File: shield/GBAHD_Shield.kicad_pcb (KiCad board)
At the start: 2 copper layers, 53.4 x 53.1 mm, 38 parts, among them J1 Conn_01x01, J10 Conn_01x10, J11 Conn_02x03_Odd_Even, J12 Conn_01x01, J2 FFC_OGBA_32, J3 FFC_GBA-SP, J4 Conn_01x16, J5 FFC_OGBA_40, J6 Conn_01x06, J7 Conn_01x08, J8 Conn_01x10, J9 Conn_01x08, Q1 Q_PMOS_GSD, SW1 SW_Push, T1 Conn_01x01, T2 Conn_01x01, T3 Conn_01x01, T4 Conn_01x01, T5 Conn_01x01, T6 Conn_01x01, T7 Conn_01x01, T8 Conn_01x01, U1 AZ1117R-ADJ, U2 74HC595, U3 74HC595, U4 SNES_7PIN, U5 ATmega328P-AU

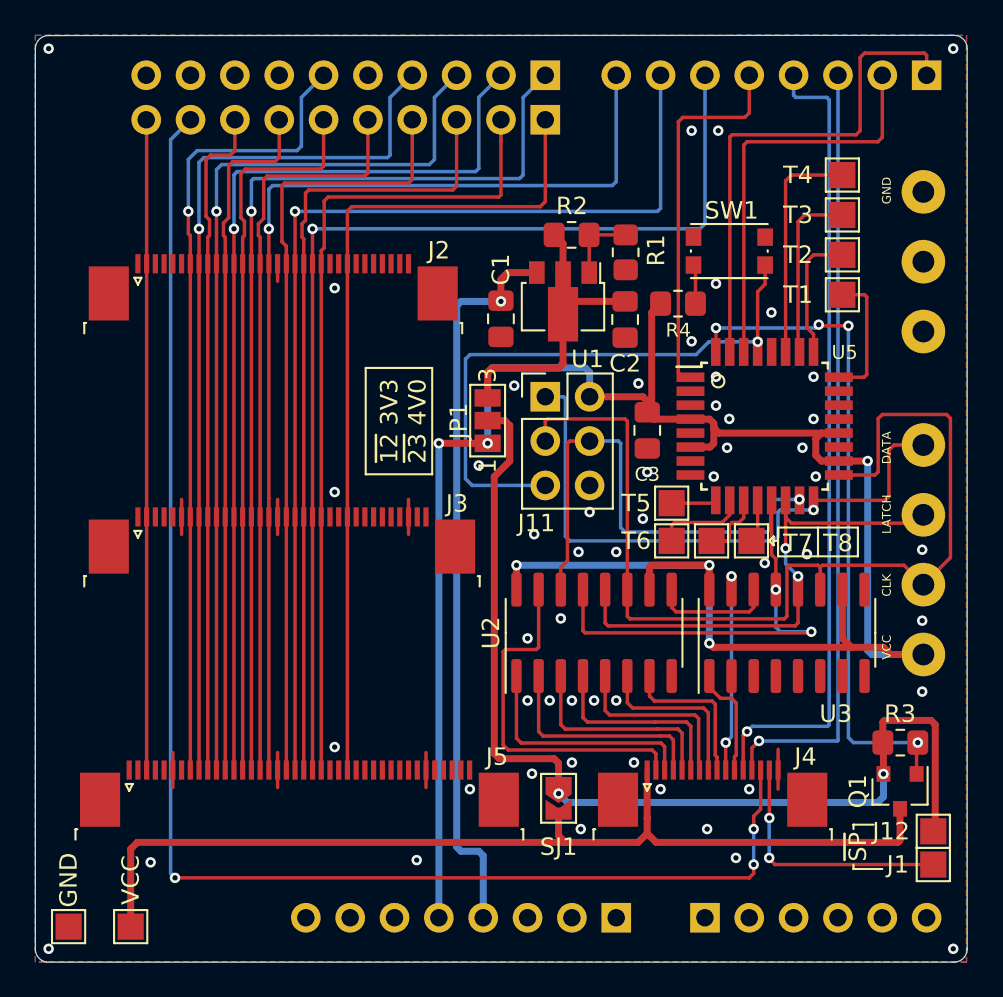
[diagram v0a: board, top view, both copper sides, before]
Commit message: Develop (#16)
* Remove get_components from Makefile, fix bluepad path

* Fixed naming of submodule

* Fixed submodule mess

* Removed bluepad32

* Re-Add Bluepad32 properly

* Update Build for adding web/bitstream handler

* Add implementation for web handler and bitstream handler

* Update arduino version

* Fix build by using bluepad template as component foundation

* Removed bluepad submodule

* Copying default component files

* Remove get_components

* Improved over all build config

* Overall refactoring and added wifi and mega handler

* Minor updates to sdkconfig

* Add first crude version to update firmware

* Remove Bluepad Debug outputs

* some cleanup

* updated .gitignore and added some files

* updated gitmodules

* fixed submodules

* Update Upgrade function

* Fix gitignore

* Fix SPIFFS upload

* a little bit of tinkering

* Changed order of run/init to be faster for TWI

* Removed endTransmission after requestFrom

* changed twi handling

* added definition for bigger I2C-Buffer

* some cleanup

* remove wifi

* Fix sending of inputs without controller available

* Fix WiFi

* fixed button mapping

* fixed button mappings and polling intervalls

* Improve Timer Code

* Refactoring and Preferences

* Add Prefs

* Add prefs

* fixed verify_flash() --> missing beginTransmission()

* Added Bluetooth Mapping, Preferences Refactoring

* Add bluetooth cfg

* Refactoring

* Remove template

* CMake fixes

* changed TWI handling - added data validity timeout

* some cleanup

* Added License Hadder

* updated CPU-flex

* Refactoring

* Beautifying

* Update Bitstream

* refactored avr-firmware to be makefile project

* added controller detection

* Better layout

* Better shield handling

* Better OTA

* For now - only load bitstream from SPIFFS to be faster

* Add Force option for ATMega update

* Added Force Option for Mega Update

* Upd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
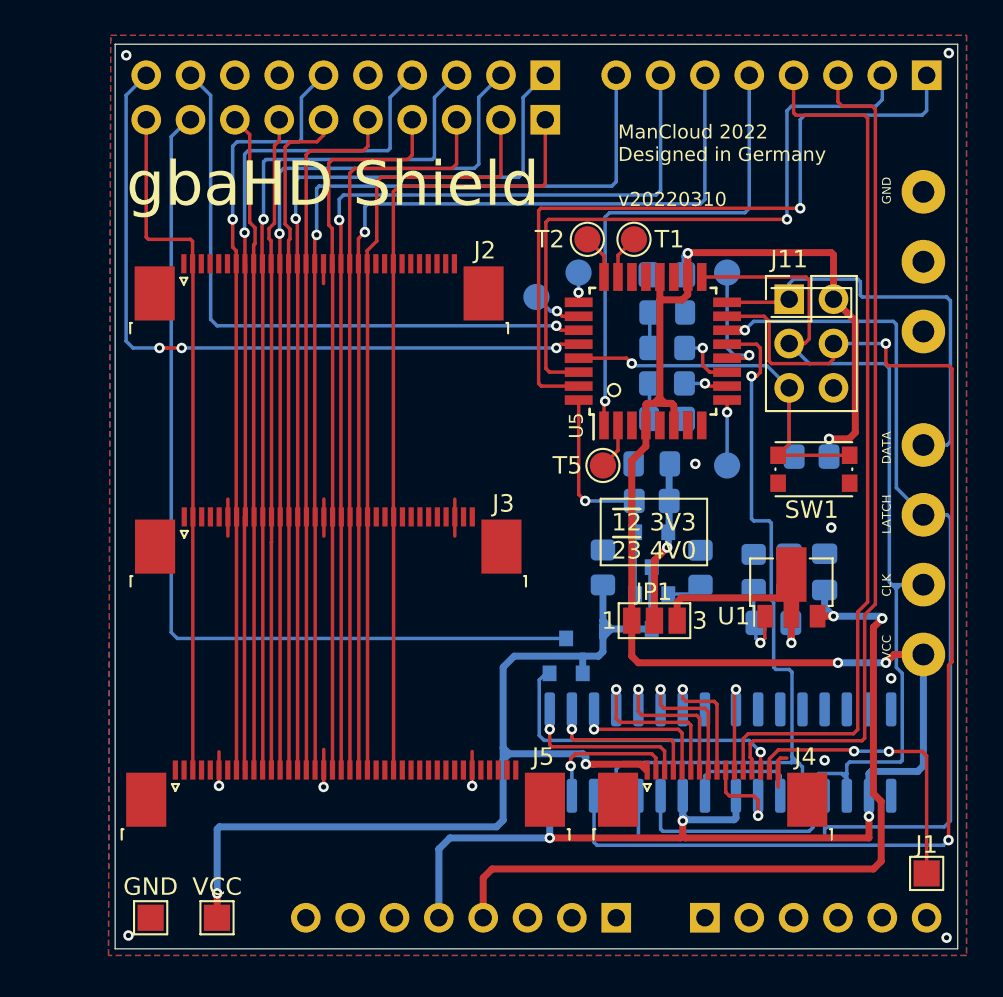
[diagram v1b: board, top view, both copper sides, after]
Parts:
- removed GND, J12, T8, VCC: Conn_01x01, TestPoint:TestPoint_Pad_1.5x1.5mm
- removed SJ1: SOLDER_JUMPER, Jumper:SolderJumper-2_P1.3mm_Open_TrianglePad1.0x1.5mm
- added C4: 47uF, Capacitor_SMD:C_0805_2012Metric_Pad1.18x1.45mm_HandSolder, B.Cu at (74.9, 51.0)
- added D1: RED, LED_SMD:LED_0805_2012Metric_Pad1.15x1.40mm_HandSolder, B.Cu at (75.8, 48.4)
- added D2: GREEN, LED_SMD:LED_0805_2012Metric_Pad1.15x1.40mm_HandSolder, B.Cu at (75.8, 42.3)
- added GND1: Conn_01x01, TestPoint:TestPoint_Pad_1.5x1.5mm, F.Cu at (46.2, 77.0)
- added Q2: Q_NMOS_GSD, Package_TO_SOT_SMD:SOT-23, B.Cu at (74.9, 59.4)
- added Q3: Q_NMOS_GSD, Package_TO_SOT_SMD:SOT-23, B.Cu at (70.0, 62.0)
- added R5: 500, Resistor_SMD:R_0805_2012Metric_Pad1.20x1.40mm_HandSolder, B.Cu at (77.7, 56.9)
- added R6: 1k, Resistor_SMD:R_0805_2012Metric_Pad1.20x1.40mm_HandSolder, B.Cu at (75.8, 46.4)
- added R7: 1k, Resistor_SMD:R_0805_2012Metric_Pad1.20x1.40mm_HandSolder, B.Cu at (75.8, 44.3)
- added R8: 10K, Resistor_SMD:R_0805_2012Metric_Pad1.20x1.40mm_HandSolder, B.Cu at (72.1, 56.9)
- added VCC1: Conn_01x01, TestPoint:TestPoint_Pad_1.5x1.5mm, F.Cu at (50.0, 77.0)
- C1, C2, C3, Q1, R1, R2, R3, R4, U2, U3: moved to B.Cu
- T1, T2, T5: footprint TestPoint:TestPoint_Pad_1.5x1.5mm -> TestPoint:TestPoint_Pad_D1.5mm
- T3, T4, T6, T7: footprint TestPoint:TestPoint_Pad_1.5x1.5mm -> TestPoint:TestPoint_Pad_D1.5mm; moved to B.Cu
- moved R2 25.1 mm to (81.9, 60.1), turned to 0 degrees
- moved C1 23.5 mm to (84.8, 57.1), turned to -90 degrees
- moved U1 21.0 mm to (82.9, 58.0), turned to 90 degrees
- moved R3 19.9 mm to (74.9, 53.1), turned to 0 degrees
- moved Q1 19.8 mm to (74.9, 55.9)
- moved R1 19.7 mm to (80.8, 57.1), turned to -90 degrees
- moved T4 18.9 mm to (68.3, 41.4)
- moved C2 17.2 mm to (82.8, 57.1), turned to -90 degrees
- moved T3 15.5 mm to (70.7, 40.0)
- moved T7 15.4 mm to (79.2, 40.0)
- moved J11 15.0 mm to (82.8, 41.5)
- moved JP1 14.9 mm to (75.1, 59.9), turned to 0 degrees
- moved T2 14.6 mm to (71.2, 38.1)
- moved SW1 13.4 mm to (84.2, 51.3), turned to 0 degrees
- moved T1 12.4 mm to (73.9, 38.1)
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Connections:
- net PIXEL_GRID renamed FPGA_COM
- net ~GBA_BUTTONS_EN~ renamed ~{GBA_BUTTONS_EN}
- J10 pad 10: (no net) -> SP_ARSCL
- J10 pad 5: (no net) -> SP_ARD12
- J10 pad 8: (no net) -> unconnected-(J10-Pad8)
- J10 pad 9: (no net) -> SP_ARSDA
- J2 pad 1: (no net) -> unconnected-(J2-Pad1)
- J2 pad 23: (no net) -> unconnected-(J2-Pad23)
- J2 pad 24: (no net) -> unconnected-(J2-Pad24)
- J2 pad 26: (no net) -> unconnected-(J2-Pad26)
- J2 pad 27: (no net) -> unconnected-(J2-Pad27)
- J2 pad 28: (no net) -> unconnected-(J2-Pad28)
- J2 pad 29: (no net) -> unconnected-(J2-Pad29)
- J2 pad 3: (no net) -> unconnected-(J2-Pad3)
- J2 pad 30: (no net) -> unconnected-(J2-Pad30)
- J2 pad 31: (no net) -> unconnected-(J2-Pad31)
- J2 pad 32: (no net) -> unconnected-(J2-Pad32)
- J2 pad 4: (no net) -> unconnected-(J2-Pad4)
- J2 pad 5: (no net) -> unconnected-(J2-Pad5)
- J2 pad 6: (no net) -> unconnected-(J2-Pad6)
- J3 pad 1: (no net) -> unconnected-(J3-Pad1)
- J3 pad 23: (no net) -> unconnected-(J3-Pad23)
- J3 pad 24: (no net) -> unconnected-(J3-Pad24)
- J3 pad 26: (no net) -> unconnected-(J3-Pad26)
- J3 pad 27: (no net) -> unconnected-(J3-Pad27)
- J3 pad 28: (no net) -> unconnected-(J3-Pad28)
- J3 pad 29: (no net) -> unconnected-(J3-Pad29)
- J3 pad 3: (no net) -> unconnected-(J3-Pad3)
- J3 pad 30: (no net) -> unconnected-(J3-Pad30)
- J3 pad 31: (no net) -> unconnected-(J3-Pad31)
- J3 pad 33: (no net) -> unconnected-(J3-Pad33)
- J3 pad 34: (no net) -> unconnected-(J3-Pad34)
- J3 pad 4: (no net) -> unconnected-(J3-Pad4)
- J3 pad 5: (no net) -> unconnected-(J3-Pad5)
- J4 pad 14: GBA_CLK -> GBA_CLK'
- J5 pad 1: (no net) -> unconnected-(J5-Pad1)
- J5 pad 2: (no net) -> unconnected-(J5-Pad2)
- J5 pad 24: (no net) -> unconnected-(J5-Pad24)
- J5 pad 25: (no net) -> unconnected-(J5-Pad25)
- J5 pad 27: (no net) -> unconnected-(J5-Pad27)
- J5 pad 28: (no net) -> unconnected-(J5-Pad28)
- J5 pad 29: (no net) -> unconnected-(J5-Pad29)
- J5 pad 30: (no net) -> unconnected-(J5-Pad30)
- J5 pad 31: (no net) -> unconnected-(J5-Pad31)
- J5 pad 32: (no net) -> unconnected-(J5-Pad32)
- J5 pad 33: (no net) -> unconnected-(J5-Pad33)
- J5 pad 34: (no net) -> unconnected-(J5-Pad34)
- J5 pad 36: (no net) -> unconnected-(J5-Pad36)
- J5 pad 37: (no net) -> unconnected-(J5-Pad37)
- J5 pad 38: (no net) -> unconnected-(J5-Pad38)
- J5 pad 39: (no net) -> unconnected-(J5-Pad39)
- J5 pad 4: (no net) -> unconnected-(J5-Pad4)
- J5 pad 40: (no net) -> unconnected-(J5-Pad40)
- J5 pad 5: (no net) -> unconnected-(J5-Pad5)
- J5 pad 7: (no net) -> unconnected-(J5-Pad7)
- J6 pad 1: (no net) -> AR_A0
- J6 pad 2: (no net) -> AR_A1
- J6 pad 3: (no net) -> AR_A2
- J6 pad 4: (no net) -> AR_A3
- J6 pad 5: (no net) -> AR_A4
- J6 pad 6: (no net) -> AR_A5
- J7 pad 1: (no net) -> SP_VIN
- J7 pad 6: (no net) -> SP_ARRES
- J7 pad 7: (no net) -> unconnected-(J7-Pad7)
- J7 pad 8: (no net) -> unconnected-(J7-Pad8)
- U3 pad 2: (no net) -> unconnected-(U3-Pad2)
- U3 pad 3: (no net) -> unconnected-(U3-Pad3)
- U3 pad 4: (no net) -> unconnected-(U3-Pad4)
- U3 pad 5: (no net) -> unconnected-(U3-Pad5)
- U3 pad 6: (no net) -> unconnected-(U3-Pad6)
- U3 pad 7: (no net) -> unconnected-(U3-Pad7)
- U3 pad 9: (no net) -> unconnected-(U3-Pad9)
- U5 pad 10: Net-(T6-Pad1) -> LED_RED
- U5 pad 11: Net-(T7-Pad1) -> LED_GREEN
- U5 pad 12: Net-(T8-Pad1) -> Net-(T7-Pad1)
- U5 pad 19: (no net) -> unconnected-(U5-Pad19)
- U5 pad 2: (no net) -> Net-(T5-Pad1)
- U5 pad 22: (no net) -> unconnected-(U5-Pad22)
- U5 pad 23: (no net) -> Net-(T1-Pad1)
- U5 pad 24: Net-(T1-Pad1) -> Net-(T2-Pad1)
- U5 pad 25: Net-(T2-Pad1) -> Net-(T3-Pad1)
- U5 pad 26: Net-(T3-Pad1) -> Net-(T4-Pad1)
- U5 pad 27: Net-(T4-Pad1) -> SP_ARSDA
- U5 pad 28: (no net) -> SP_ARSCL
- U5 pad 7: (no net) -> unconnected-(U5-Pad7)
- U5 pad 8: (no net) -> unconnected-(U5-Pad8)
- U5 pad 9: Net-(T5-Pad1) -> Net-(T6-Pad1)
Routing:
- net VCC: track 57.9 -> 9.35 mm, vias 2 -> 1
- net SP_ARSCL: track 0.00 -> 41.9 mm, vias 0 -> 3
- net ICSP_MOSI: track 28.6 -> 67.9 mm, vias 1 -> 2
- net SP_ARSDA: track 0.00 -> 35.8 mm, vias 0 -> 1
- net SNS_LATCH: track 29.7 -> 63.4 mm, vias 2 -> 1
- net GBA_CLK: track 83.3 -> 52.7 mm, vias 3 -> 0
- net GBA_POWER_SEL: track 38.6 -> 14.1 mm, vias 4 -> 1
- net GBA_CLK': track 0.00 -> 18.0 mm, vias 0 -> 1
- net ~{GBA_BUTTONS_EN}: track 25.0 -> 42.7 mm, vias 2 -> 1
- net SP_ARD1: track 23.6 -> 37.6 mm, vias 0 -> 1
- net GBA_UP: track 20.7 -> 7.95 mm, vias 0 -> 1
- net RX: track 29.3 -> 41.9 mm, vias 0 -> 1
- net AT_RST: track 36.1 -> 25.0 mm
- net Net-(T4-Pad1): track 13.2 -> 2.88 mm, vias 0 -> 1
- net ICSP_MISO: track 34.1 -> 24.5 mm, vias 1 -> 0
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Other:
- board size 53.4 x 53.1 mm -> 48.3 x 51.8 mm
- net class Default removed
- net class VCC removed
- board text added: "ManCloud 2022 Designed in Germany v20220310"
- board text added: "~{12} 3V3 ~{23} 4V0"
- board text removed: "ManCloud 2021 Designed in Germany v20210416"
- board text removed: "~12~ 3V3 ~23~ 4V0"
- board text removed: "~SP~"
